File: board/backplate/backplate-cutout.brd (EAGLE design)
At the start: 128 x 43 mm, 0 parts

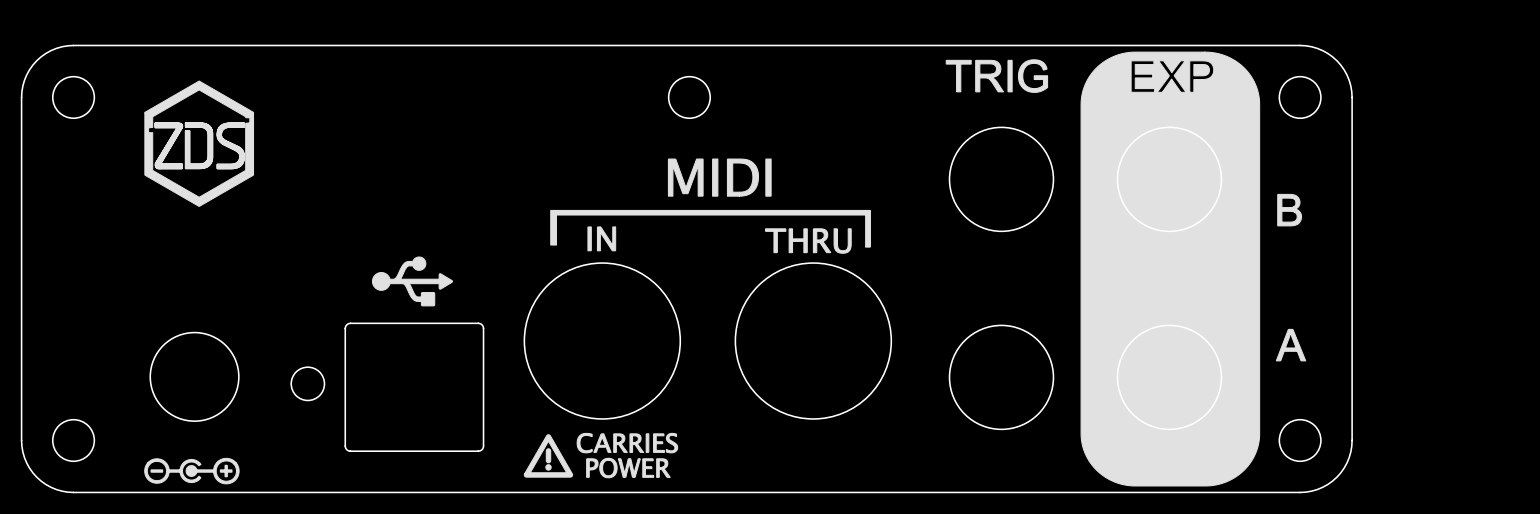
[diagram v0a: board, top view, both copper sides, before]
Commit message: board changes
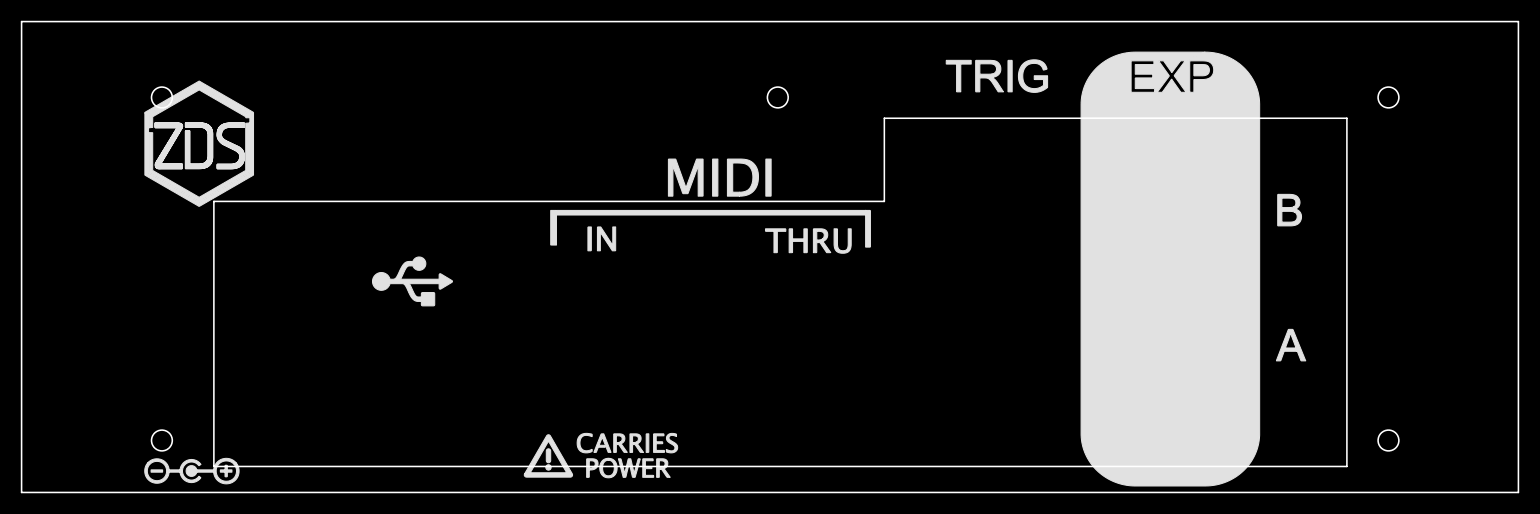
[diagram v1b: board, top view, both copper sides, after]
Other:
- board size 128 x 43 mm -> 144 x 45.3 mm
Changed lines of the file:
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@@
 <layer number="19" name="Unrouted" color="6" fill="1" visible="yes" active="yes"/>
 <layer number="20" name="Dimension" color="24" fill="1" visible="yes" active="yes"/>
-<layer number="21" name="tPlace" color="7" fill="1" visible="yes" active="yes"/>
-<layer number="22" name="bPlace" color="7" fill="1" visible="yes" active="yes"/>
+<layer number="21" name="tPlace" color="7" fill="1" visible="no" active="yes"/>
+<layer number="22" name="bPlace" color="7" fill="1" visible="no" active="yes"/>
 <layer number="23" name="tOrigins" color="15" fill="1" visible="yes" active="yes"/>
 <layer number="24" name="bOrigins" color="15" fill="1" visible="yes" active="yes"/>
@@
 </layers>
 <board>
+<fusionsync huburn="a.cGVyc29uYWw6dWUyYjI3ZGMz" projecturn="a.cGVyc29uYWw6dWUyYjI3ZGMzIzIwMjAwOTA3MzMwMzQ5MzAx" f3durn="urn:adsk.wipprod:dm.lineage:F2SyIyUDRYKL4E1-pcYrKg" pcbguid="b63c4ac4-db3a-470d-925e-3112f8fd1903" lastpulledtime="" lastsyncedchangeguid="" latestrevisionid="956b5319-7c00-45dc-8160-7c84e59f1625" lastsyncedrevisionid="956b5319-7c00-45dc-8160-7c84e59f1625" lastboardhashguid="3e991383-107f-c271-2332-597896a6ed77" lastpushedtime="2020-11-01T21:22:31Z" linktopcb3d="true"/>
 <plain>
-<wire x1="5" y1="43" x2="123" y2="43" width="0.1524" layer="20"/>
-<wire x1="123" y1="43" x2="128" y2="38" width="0.1524" layer="20" curve="-90"/>
-<wire x1="128" y1="38" x2="128" y2="5" width="0.1524" layer="20"/>
-<wire x1="128" y1="5" x2="123" y2="0" width="0.1524" layer="20" curve="-90"/>
-<wire x1="123" y1="0" x2="5" y2="0" width="0.1524" layer="20"/>
-<wire x1="5" y1="0" x2="0" y2="5" width="0.1524" layer="20" curve="-90"/>
-<wire x1="0" y1="5" x2="0" y2="38" width="0.1524" layer="20"/>
-<wire x1="0" y1="38" x2="5" y2="43" width="0.1524" layer="20" curve="-90"/>
-<circle x="16.64" y="11.12" radius="4.26" width="0.1524" layer="20"/>
-<circle x="27.54" y="10.45" radius="1.6" width="0.1524" layer="20"/>
-<circle x="55.87" y="14.57" radius="7.5" width="0.1524" layer="20"/>
-<circle x="76.17" y="14.57" radius="7.5" width="0.1524" layer="20"/>
-<circle x="94.27" y="11.07" radius="5" width="0.1524" layer="20"/>
-<circle x="110.43" y="11.07" radius="5" width="0.1524" layer="20"/>
-<circle x="94.27" y="30.12" radius="5" width="0.1524" layer="20"/>
-<wire x1="43.94" y1="3.97" x2="31.64" y2="3.97" width="0.1524" layer="20"/>
-<wire x1="31.64" y1="3.97" x2="31.14" y2="4.47" width="0.1524" layer="20" curve="-90"/>
-<wire x1="31.14" y1="4.47" x2="31.14" y2="15.77" width="0.1524" layer="20"/>
-<wire x1="31.14" y1="15.77" x2="31.64" y2="16.27" width="0.1524" layer="20" curve="-90"/>
-<wire x1="31.64" y1="16.27" x2="43.94" y2="16.27" width="0.1524" layer="20"/>
-<wire x1="43.94" y1="16.27" x2="44.44" y2="15.77" width="0.1524" layer="20" curve="-90"/>
-<wire x1="44.44" y1="15.77" x2="44.44" y2="4.47" width="0.1524" layer="20"/>
-<wire x1="44.44" y1="4.47" x2="43.94" y2="3.97" width="0.1524" layer="20" curve="-90"/>
-<circle x="5" y="38" radius="2" width="0.1524" layer="20"/>
-<circle x="123" y="38" radius="2" width="0.1524" layer="20"/>
-<circle x="123" y="5" radius="2" width="0.1524" layer="20"/>
-<circle x="5" y="5" radius="2" width="0.1524" layer="20"/>
-<circle x="64.25" y="38" radius="2" width="0.1524" layer="20"/>
-<circle x="110.43" y="30.12" radius="5" width="0.1524" layer="20"/>
+<wire x1="18.5" y1="28" x2="83" y2="28" width="0.1524" layer="20"/>
+<wire x1="83" y1="28" x2="83" y2="36" width="0.1524" layer="20"/>
+<wire x1="83" y1="36" x2="127.5" y2="36" width="0.1524" layer="20"/>
+<wire x1="127.5" y1="36" x2="127.5" y2="2.5" width="0.1524" layer="20"/>
+<wire x1="127.5" y1="2.5" x2="18.5" y2="2.5" width="0.1524" layer="20"/>
+<wire x1="18.5" y1="2.5" x2="18.5" y2="28" width="0.1524" layer="20"/>
+<circle x="13.5" y="38" radius="1" width="0.1524" layer="20"/>
+<circle x="131.5" y="38" radius="1" width="0.1524" layer="20"/>
+<circle x="131.5" y="5" radius="1" width="0.1524" layer="20"/>
+<circle x="13.5" y="5" radius="1" width="0.1524" layer="20"/>
+<circle x="72.75" y="38" radius="1" width="0.1524" layer="20"/>
 <polygon width="0.1" layer="21">
 <vertex x="16.34705625" y="2.580871875"/>
@@
 <text x="115" y="39" size="1.778" layer="22" rot="MR0">ZDS Shifter Pro REV: A</text>
 <text x="83" y="39" size="1.778" layer="22" rot="MR0">10/20/2020</text>
+<wire x1="0" y1="45.3" x2="144" y2="45.3" width="0.1524" layer="20"/>
+<wire x1="144" y1="45.3" x2="144" y2="0" width="0.1524" layer="20"/>
+<wire x1="144" y1="0" x2="0" y2="0" width="0.1524" layer="20"/>
+<wire x1="0" y1="0" x2="0" y2="45.3" width="0.1524" layer="20"/>
 </plain>
 <attributes>
@@
 </board>
 </drawing>
+<compatibility>
+<note version="8.3" severity="warning">
+Since Version 8.3, EAGLE supports Fusion synchronisation.
+This feature will not be available in this version and saving
+the document will break the link to the Fusion PCB feature.
+</note>
+</compatibility>
 </eagle>
